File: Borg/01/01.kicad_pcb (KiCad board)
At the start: 2 copper layers, 98.7 x 98.6 mm, 2 parts

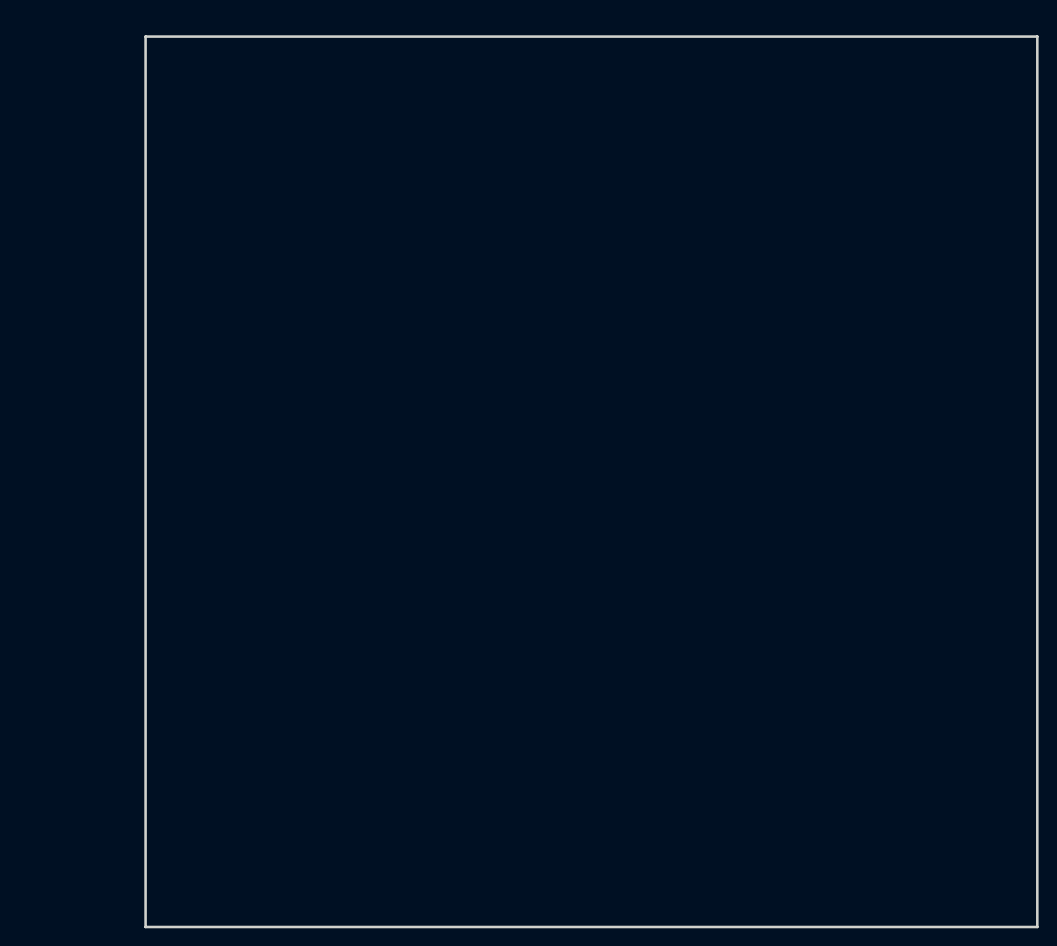
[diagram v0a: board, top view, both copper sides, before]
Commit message: Updates
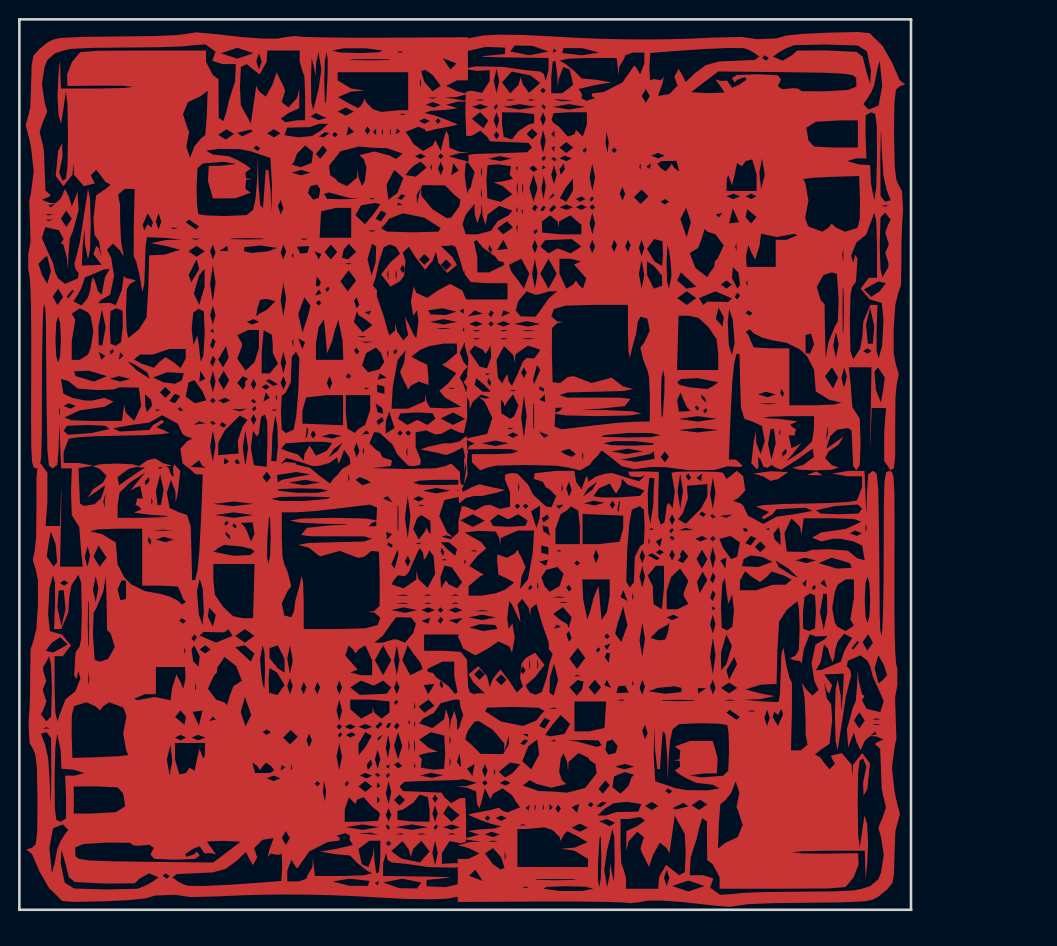
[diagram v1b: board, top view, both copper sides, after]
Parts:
- removed the svg2mod at (214.0, 91.4)
- added svg2mod: G***, borg:Borg.Cu.01, F.Cu at (103.0, 75.4)
- added svg2mod: G***, borg:Borg.Cu.02, F.Cu at (151.2, 75.6)
- added svg2mod: G***, borg:Borg.Cu.01, F.Cu at (150.5, 123.8)
- added svg2mod: G***, borg:Borg.Cu.02, F.Cu at (102.9, 123.1)
- moved svg2mod 14.1 mm to (127.0, 99.1)
